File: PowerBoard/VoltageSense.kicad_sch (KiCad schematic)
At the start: 24 parts

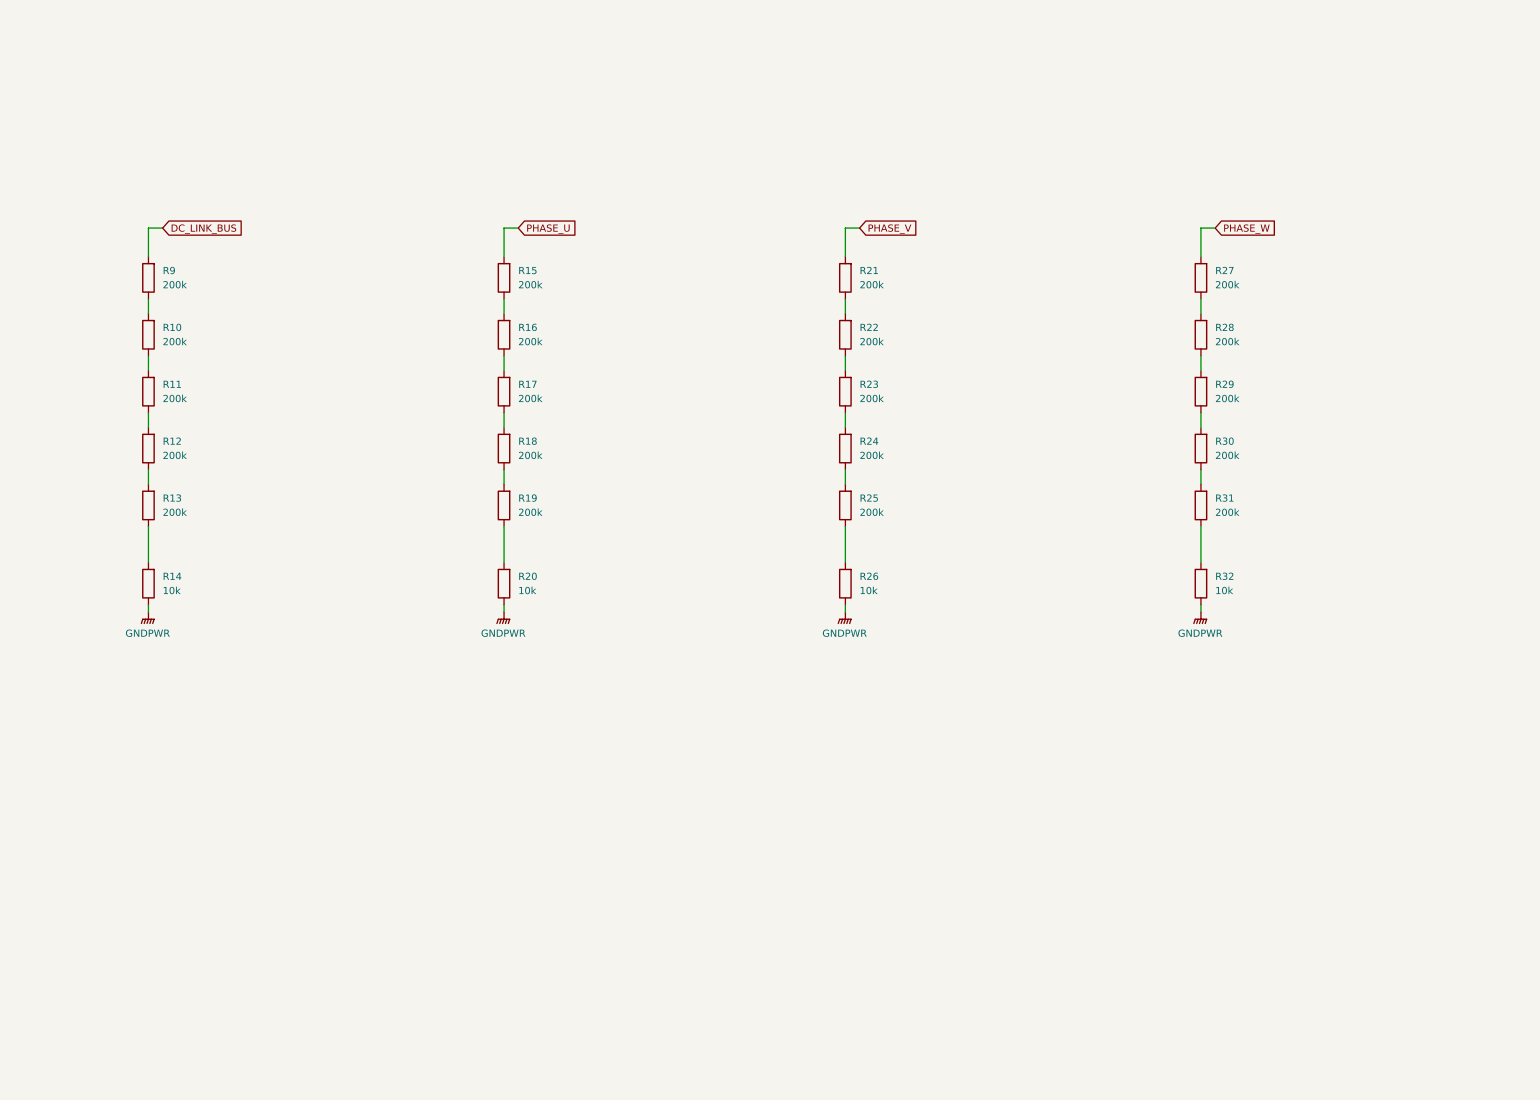
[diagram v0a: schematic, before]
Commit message: u
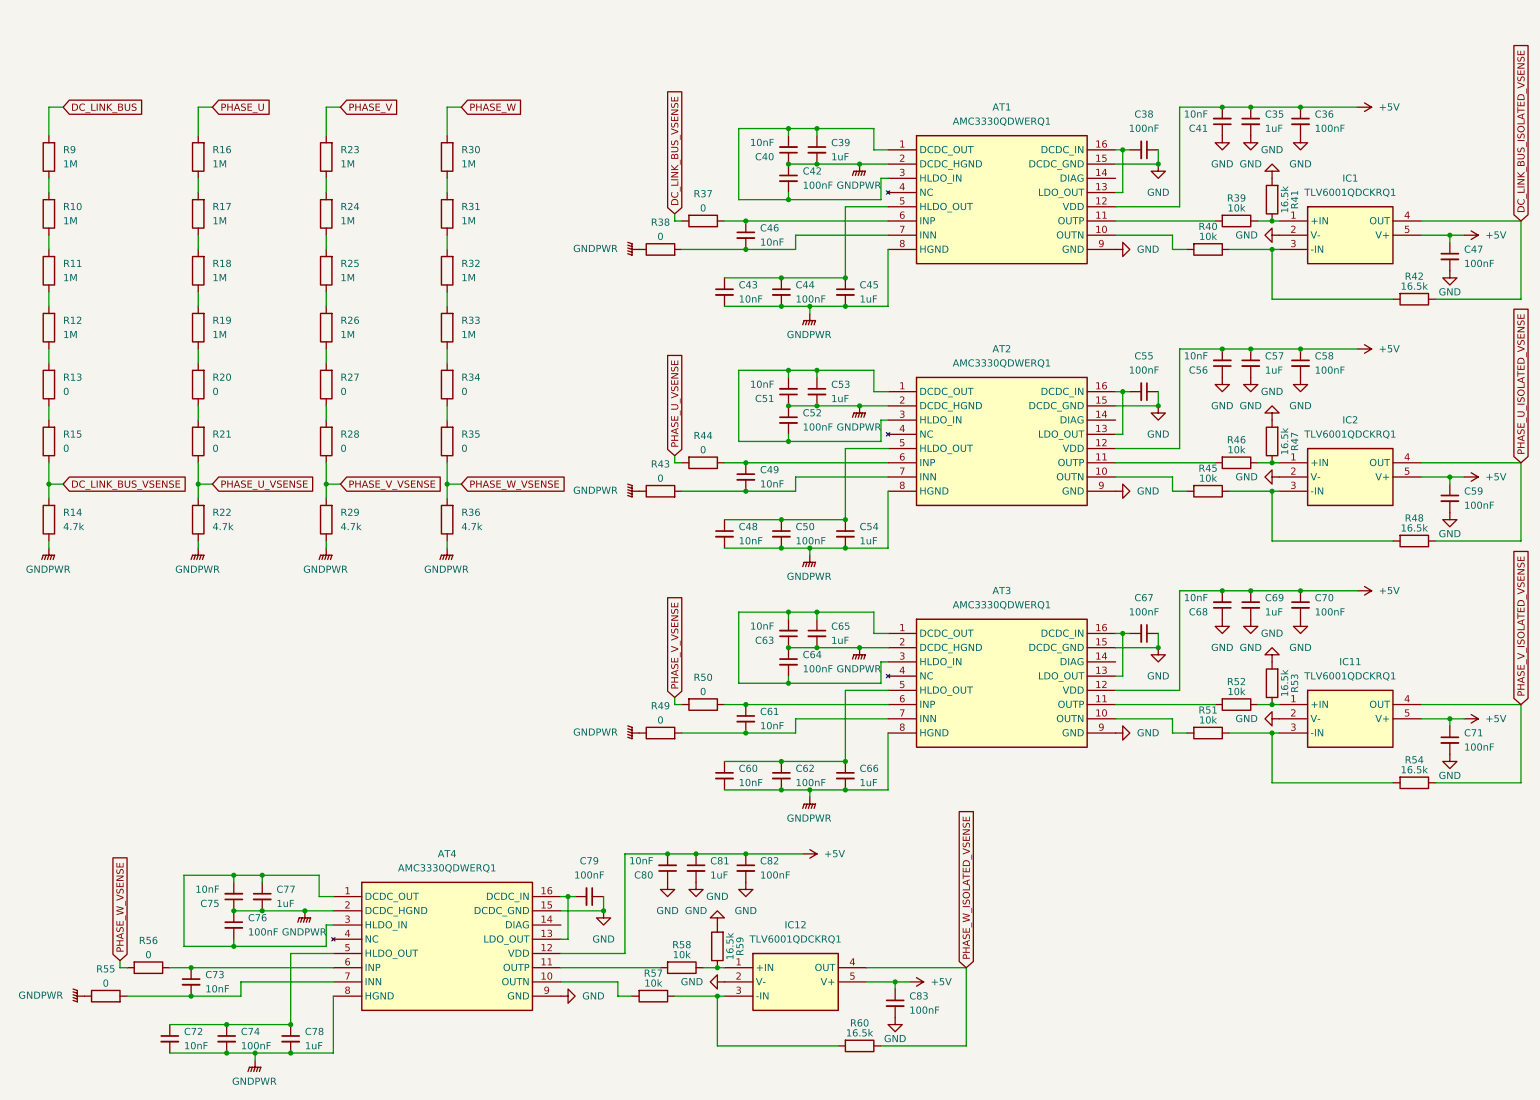
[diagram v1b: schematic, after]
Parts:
- added AT1, AT2, AT3, AT4: AMC3330QDWERQ1, SOIC127P1030X265-16N, symbol InverterCom:AMC3330QDWERQ1
- added C35, C39, C45, C53, C54, C57, C65, C66, C69, C77, C78, C81: 1uF, Capacitor_SMD:C_1210_3225Metric_Pad1.33x2.70mm_HandSolder, symbol Device:C_Small
- added C36, C38, C42, C44, C47, C50, C52, C55, C58, C59, C62, C64, C67, C70, C71, C74, C76, C79, C82, C83: 100nF, Capacitor_SMD:C_1210_3225Metric_Pad1.33x2.70mm_HandSolder, symbol Device:C_Small
- added C40, C41, C43, C46, C48, C49, C51, C56, C60, C61, C63, C68, C72, C73, C75, C80: 10nF, Capacitor_SMD:C_1210_3225Metric_Pad1.33x2.70mm_HandSolder, symbol Device:C_Small
- added IC1, IC11, IC12, IC2: TLV6001QDCKRQ1, InverterCom:SOT65P210X110-5N, symbol InverterCom:TLV6001QDCKRQ1
- added R33: 1M, Resistor_SMD:R_1210_3225Metric_Pad1.30x2.65mm_HandSolder, symbol Device:R
- added R34, R35, R37, R38, R43, R44, R49, R50, R55, R56: 0, Resistor_SMD:R_1210_3225Metric_Pad1.30x2.65mm_HandSolder, symbol Device:R
- added R36: 4.7k, Resistor_SMD:R_1210_3225Metric_Pad1.30x2.65mm_HandSolder, symbol Device:R
- added R39, R40, R45, R46, R51, R52, R57, R58: 10k, Resistor_SMD:R_1210_3225Metric_Pad1.30x2.65mm_HandSolder, symbol Device:R
- added R41, R42, R47, R48, R53, R54, R59, R60: 16.5k, Resistor_SMD:R_1210_3225Metric_Pad1.30x2.65mm_HandSolder, symbol Device:R
- R10, R11, R12, R16, R17, R18, R19, R23, R24, R25, R30, R31, R9: value 200k -> 1M; footprint 1210 -> Resistor_SMD:R_1210_3225Metric_Pad1.30x2.65mm_HandSolder
- R13, R15, R21, R27, R28: value 200k -> 0; footprint 1210 -> Resistor_SMD:R_1210_3225Metric_Pad1.30x2.65mm_HandSolder
- R14: value 10k -> 4.7k; footprint 1210 -> Resistor_SMD:R_1210_3225Metric_Pad1.30x2.65mm_HandSolder
- R20: value 10k -> 0; footprint 1210 -> Resistor_SMD:R_1210_3225Metric_Pad1.30x2.65mm_HandSolder
- R22, R29: value 200k -> 4.7k; footprint 1210 -> Resistor_SMD:R_1210_3225Metric_Pad1.30x2.65mm_HandSolder
- R26, R32: value 10k -> 1M; footprint 1210 -> Resistor_SMD:R_1210_3225Metric_Pad1.30x2.65mm_HandSolder
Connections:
- net GNDPWR: now also R22.1, R29.1, AT1.2 (DCDC_HGND), AT1.8 (HGND), AT2.2 (DCDC_HGND), AT2.8 (HGND), AT3.2 (DCDC_HGND), AT3.8 (HGND), AT4.2 (DCDC_HGND), AT4.8 (HGND), C39.2, C40.1, C42.1, C43.2, C44.2, C45.2, C48.2, C50.2, C51.1, C52.1, C53.2, C54.2, C60.2, C62.2, C63.1, C64.1, C65.2, C66.2, C72.2, C74.2, C75.1, C76.1, C77.2, C78.2, R36.1, R38.1, R43.1, R49.1, R55.1; no longer R20.1, R26.1, R32.1
- net PHASE_U: now also R16.2; no longer R15.2
- net PHASE_V: now also R23.2; no longer R21.2
- net PHASE_W: now also R30.2; no longer R27.2
- net PHASE_V_VSENSE: now reaches R28.1, R29.2
- net PHASE_V_VSENSE: now also R50.2
- net at R13.1: now also R15.2; no longer R14.2
- net DC_LINK_BUS_VSENSE: now reaches R15.1
- net DC_LINK_BUS_VSENSE: now also R14.2, R37.2; no longer R16.2
- net PHASE_U_VSENSE: now reaches R21.1, R22.2
- net PHASE_U_VSENSE: now also R44.2
- new net: AT4.5 (HLDO_OUT), C72.1, C74.1, C78.1
- new net: IC1.1 (+IN), R39.1, R41.1
- new net: IC1.3 (-IN), R40.1, R42.2
- new net: AT1.1 (DCDC_OUT), AT1.3 (HLDO_IN), C39.1, C40.2, C42.2
- new net: AT1.10 (OUTN), R40.2
- new net: AT1.11 (OUTP), R39.2
- new net: AT1.13 (LDO_OUT), AT1.16 (DCDC_IN), C38.2
- new net: AT1.5 (HLDO_OUT), C43.1, C44.1, C45.1
- new net: AT1.6 (INP), C46.1, R37.1
- new net: AT1.7 (INN), C46.2, R38.2
- new net: R20.1, R21.2
- new net: R33.1, R34.2
- new net: R32.1, R33.2
- new net: IC11.3 (-IN), R51.1, R54.2
- new net: AT3.10 (OUTN), R51.2
- new net: AT2.1 (DCDC_OUT), AT2.3 (HLDO_IN), C51.2, C52.2, C53.1
- new net: AT3.7 (INN), C61.2, R49.2
- new net: R34.1, R35.2
- new net: AT2.5 (HLDO_OUT), C48.1, C50.1, C54.1
- new net: AT3.1 (DCDC_OUT), AT3.3 (HLDO_IN), C63.2, C64.2, C65.1
- new net: AT3.11 (OUTP), R52.2
- new net: AT3.13 (LDO_OUT), AT3.16 (DCDC_IN), C67.2
- new net: AT3.5 (HLDO_OUT), C60.1, C62.1, C66.1
- new net: AT3.6 (INP), C61.1, R50.1
- new net: R26.1, R27.2
- new net: AT4.6 (INP), C73.1, R56.1
- new net: AT4.7 (INN), C73.2, R55.2
- new net: IC11.1 (+IN), R52.1, R53.1
- new net: AT4.1 (DCDC_OUT), AT4.3 (HLDO_IN), C75.2, C76.2, C77.1
- new net: AT4.10 (OUTN), R57.2
- new net: AT4.11 (OUTP), R58.2
- new net: AT4.13 (LDO_OUT), AT4.16 (DCDC_IN), C79.2
- new net: AT2.10 (OUTN), R45.2
- new net: AT2.11 (OUTP), R46.2
- new net: AT2.13 (LDO_OUT), AT2.16 (DCDC_IN), C55.2
- new net: AT2.6 (INP), C49.1, R44.1
- new net: AT2.7 (INN), C49.2, R43.2
- new net: IC12.1 (+IN), R58.1, R59.1
- new net: IC12.3 (-IN), R57.1, R60.2
- new net: IC2.1 (+IN), R46.1, R47.1
- new net: IC2.3 (-IN), R45.1, R48.2
- new net +5V: AT1.12 (VDD), AT2.12 (VDD), AT3.12 (VDD), AT4.12 (VDD), C35.1, C36.1, C41.2, C47.1, C56.2, C57.1, C58.1, C59.1, C68.2, C69.1, C70.1, C71.1, C80.2, C81.1, C82.1, C83.1, IC1.5 (V+), IC11.5 (V+), IC12.5 (V+), IC2.5 (V+)
- new net DC_LINK_BUS_ISOLATED_VSENSE: IC1.4 (OUT), R42.1
- new net GND: AT1.15 (DCDC_GND), AT1.9 (GND), AT2.15 (DCDC_GND), AT2.9 (GND), AT3.15 (DCDC_GND), AT3.9 (GND), AT4.15 (DCDC_GND), AT4.9 (GND), C35.2, C36.2, C38.1, C41.1, C47.2, C55.1, C56.1, C57.2, C58.2, C59.2, C67.1, C68.1, C69.2, C70.2, C71.2, C79.1, C80.1, C81.2, C82.2, C83.2, IC1.2 (V-), IC11.2 (V-), IC12.2 (V-), IC2.2 (V-), R41.2, R47.2, R53.2, R59.2
- new net PHASE_U_ISOLATED_VSENSE: IC2.4 (OUT), R48.1
- new net PHASE_V_ISOLATED_VSENSE: IC11.4 (OUT), R54.1
- new net PHASE_W_ISOLATED_VSENSE: IC12.4 (OUT), R60.1
- new net PHASE_W_VSENSE: R35.1, R36.2, R56.2
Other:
- moved on the sheet: R14, R9

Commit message: vsense
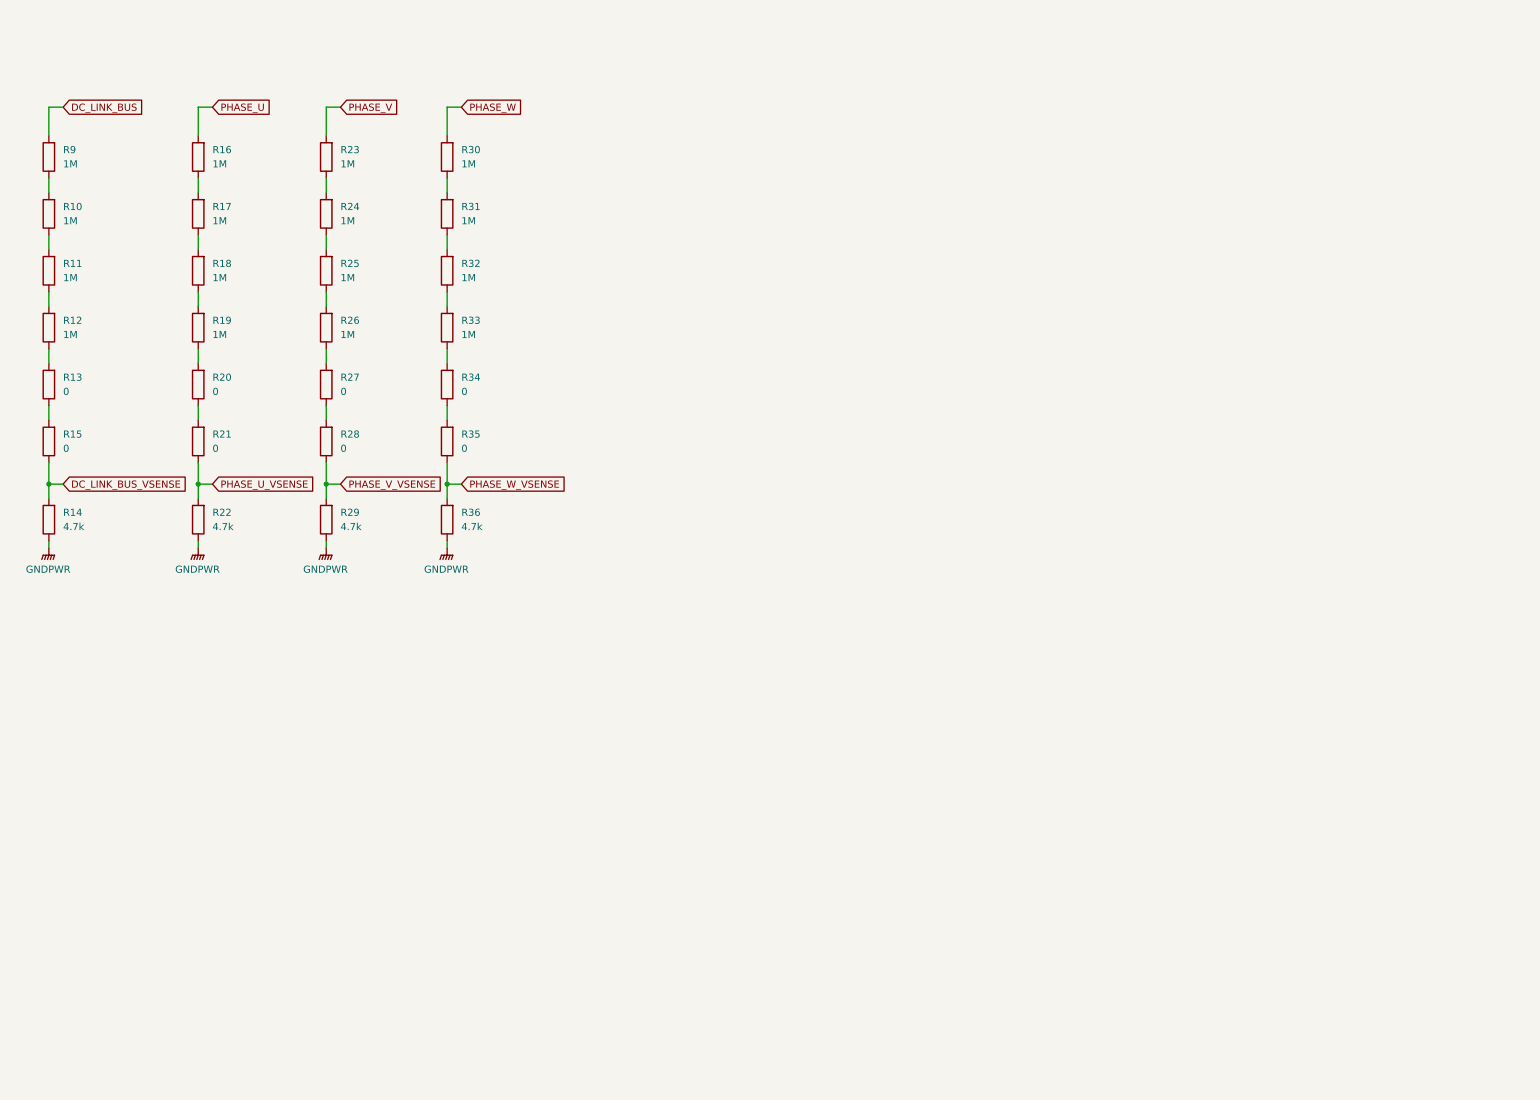
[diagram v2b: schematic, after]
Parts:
- removed AT1, AT2, AT3, AT4: AMC3330QDWERQ1, SOIC127P1030X265-16N, symbol InverterCom:AMC3330QDWERQ1
- removed C35, C39, C45, C53, C54, C57, C65, C66, C69, C77, C78, C81: 1uF, Capacitor_SMD:C_1210_3225Metric_Pad1.33x2.70mm_HandSolder, symbol Device:C_Small
- removed C36, C38, C42, C44, C47, C50, C52, C55, C58, C59, C62, C64, C67, C70, C71, C74, C76, C79, C82, C83: 100nF, Capacitor_SMD:C_1210_3225Metric_Pad1.33x2.70mm_HandSolder, symbol Device:C_Small
- removed C40, C41, C43, C46, C48, C49, C51, C56, C60, C61, C63, C68, C72, C73, C75, C80: 10nF, Capacitor_SMD:C_1210_3225Metric_Pad1.33x2.70mm_HandSolder, symbol Device:C_Small
- removed IC1, IC11, IC12, IC2: TLV6001QDCKRQ1, InverterCom:SOT65P210X110-5N, symbol InverterCom:TLV6001QDCKRQ1
- removed R37, R38, R43, R44, R49, R50, R55, R56: 0, Resistor_SMD:R_1210_3225Metric_Pad1.30x2.65mm_HandSolder, symbol Device:R
- removed R39, R40, R45, R46, R51, R52, R57, R58: 10k, Resistor_SMD:R_1210_3225Metric_Pad1.30x2.65mm_HandSolder, symbol Device:R
- removed R41, R42, R47, R48, R53, R54, R59, R60: 16.5k, Resistor_SMD:R_1210_3225Metric_Pad1.30x2.65mm_HandSolder, symbol Device:R
